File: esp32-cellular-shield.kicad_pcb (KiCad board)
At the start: 2 copper layers, 68.5 x 53.3 mm, 63 parts, among them J2 CONN_01X05, Q1 Q_NPN_BEC, Q2 Q_NPN_BEC, Q3 Q_NPN_BEC, Q4 Q_PMOS_GSD, SW1 SW_Push, U1 SIM_HOLDER, U2 SIM800C, U3 Ra-02, U4 MCP601OT, U6 MCP16311-MNY, U7 TC1264-3.3VAB

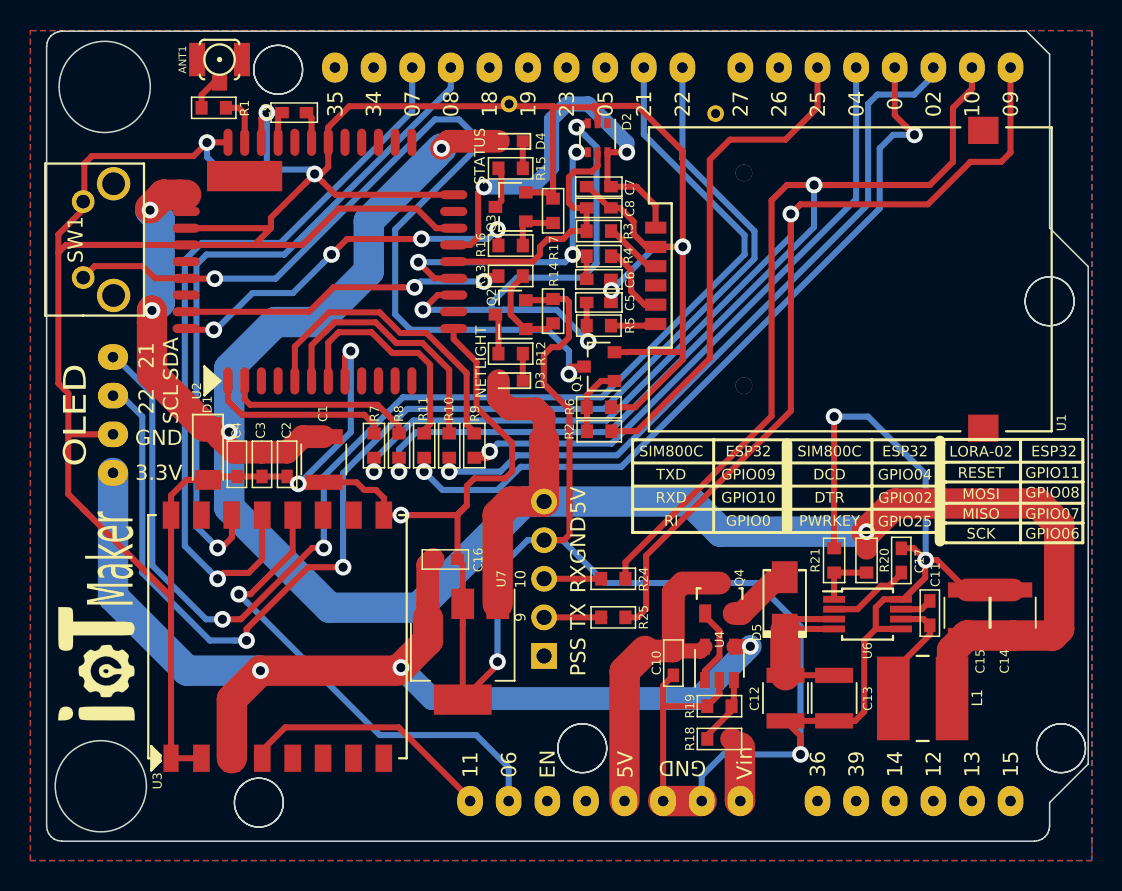
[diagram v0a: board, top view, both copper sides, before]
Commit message: modifypinout sample esp32-uno
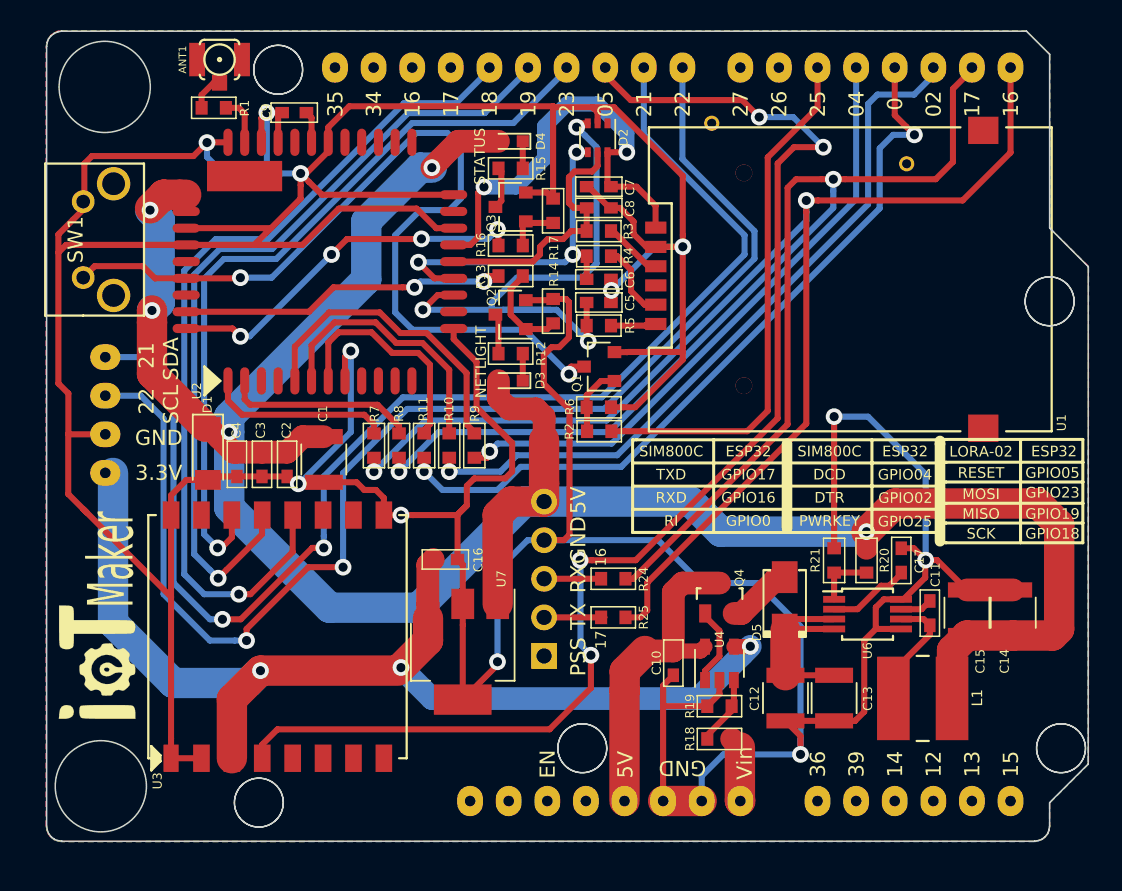
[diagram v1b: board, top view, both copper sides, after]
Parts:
- removed the REF** at (139.4, 55.6)
- removed the REF** at (153.0, 56.3)
- added REF**: SolderWirePad_single_1mmDrill, Wire_Pads:SolderWirePad_single_1mmDrill, F.Cu at (152.8, 56.9)
- added REF**: SolderWirePad_single_1mmDrill, Wire_Pads:SolderWirePad_single_1mmDrill, F.Cu at (165.6, 59.6)
- Q4: value Q_PMOS_GSD -> AO3401_PMOS_GSD
- moved G*** 0.11 mm to (112.3, 92.4)
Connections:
- S1 pad 1: RA_RESET -> (no net)
- S1 pad 2: RA_SCK -> (no net)
- S1 pad 25: (no net) -> RA_RESET
- S1 pad 26: (no net) -> RA_MOSI/SPID
- S1 pad 27: (no net) -> RA_MISO/SPIQ
- S1 pad 28: (no net) -> RA_SCK
- S1 pad 29: RA_MOSI/SPID -> (no net)
- S1 pad 30: RA_MISO/SPIQ -> (no net)
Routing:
- net RA_RESET: track 16.9 -> 86.6 mm, vias 0 -> 4
- net RA_SCK: track 31.8 -> 56.9 mm
- net RA_MOSI/SPID: track 44.9 -> 50.5 mm
- net RA_MISO/SPIQ: track 50.1 -> 53.7 mm
- net SIM800C_PWRKEY: track 60.6 -> 58.2 mm
- net PWRKEY: track 32.7 -> 34.8 mm
- net +3V3: track 70.1 -> 71.8 mm
- net GND: track 416.5 -> 414.9 mm
- net VDD: track 169.4 -> 167.8 mm
- net GPS_TX: track 90.3 -> 91.2 mm
- net SDA: track 83.0 -> 83.9 mm
- net SCL: track 83.9 -> 84.7 mm
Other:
- net class Default: clearance 0.1 -> 0.254
- rule trace_clearance: 0.1 -> 0.254
- board text added: "16"
- board text added: "17"
- board text added: "GPIO16"
- board text added: "GPIO17"
- board text removed: "06"
- board text removed: "07"
- board text removed: "08"
- board text removed: "09"
- board text removed: "10"
- board text removed: "11"
- board text removed: "9"
- board text removed: "GPIO07"
- board text removed: "GPIO08"
- board text removed: "GPIO09"
- board text removed: "GPIO10"
- board text removed: "OLED"
